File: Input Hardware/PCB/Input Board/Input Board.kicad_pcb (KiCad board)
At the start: 2 copper layers, 255 x 180 mm, 458 parts, among them J1601 1.71" SSD1312 OLED, J901 USB_C_Receptacle_USB2.0_16P, SW1501 Rotary encoder, SW1502 Rotary encoder, U1101 74HCS95, U1102 DRV8837, U1103 DRV8837, U1104 DRV8837, U1105 DRV8837, U1201 74HCS95, U1202 DRV8837, U1203 DRV8837, U1204 DRV8837, U1205 DRV8837, U1301 74HCS95, U1302 DRV8837, U1303 DRV8837, U1304 DRV8837, U1305 DRV8837, U1401 74HCS95, U1402 DRV8837, U1403 DRV8837, U1404 DRV8837, U1405 DRV8837, U1501 74HC595, U1701 LM317_TO-252, U1702 LM317_TO-252, U301 ADA4891, U302 ADA4891, U401 ADA4891, U402 ADA4891, U501 ADA4891, U502 ADA4891, U601 ADA4891, U602 ADA4891, U701 ADA4891, U702 CD4051B, U703 CD4051B, U801 ADA4891, U802 CD4051B, U803 CD4051B, U901 USBLC6-2SC6, U902 STM32F303RBTx, Y901 ECS-2520MV-xxx-xx

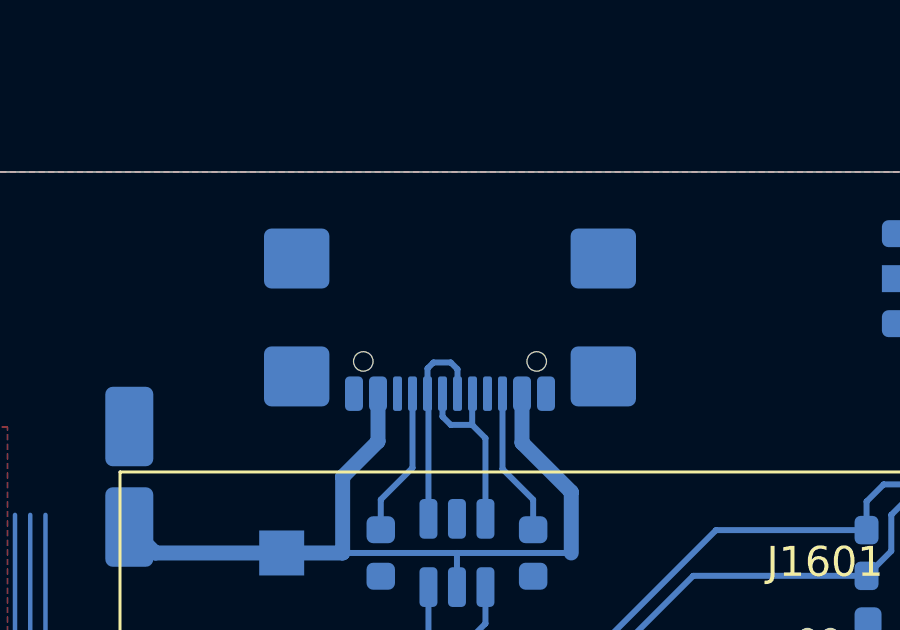
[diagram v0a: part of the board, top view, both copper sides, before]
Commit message: minor schematic changes and value assignment
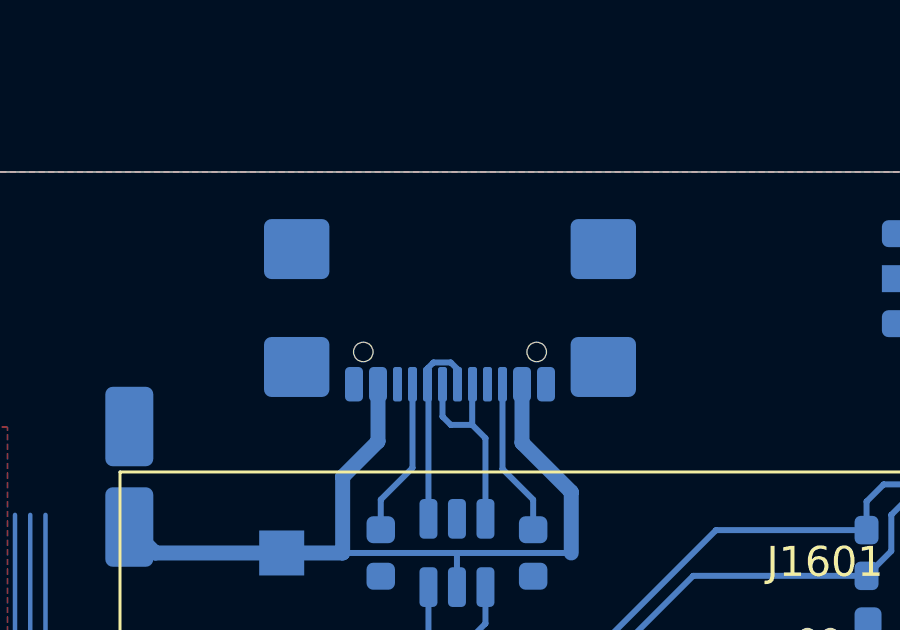
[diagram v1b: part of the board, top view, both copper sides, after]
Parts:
- moved J901 0.31 mm to (255.0, 53.4)
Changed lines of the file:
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@@
 	(footprint "Connector_USB:USB_C_Receptacle_GCT_USB4110"
 		(layer "B.Cu")
-		(at 255 53.71)
+		(at 255 53.395)
 		(descr "USB 2.0 Type C Receptacle, GCT, 16P, top mounted, horizontal, 5A, https://gct.co/files/drawings/usb4110.pdf")
 		(tags "USB 2.0 C Type-C Receptacle SMD 16P 16C USB4110-GF-A")
